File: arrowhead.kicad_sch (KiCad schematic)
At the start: 148 parts, among them J1 USB_C_Receptacle_USB2.0_14P, J2 USB_C_Receptacle_USB2.0_14P, J3 USB3_A, J4 USB3_A, U1 TUSB2046BVF, Y1 Crystal_GND23

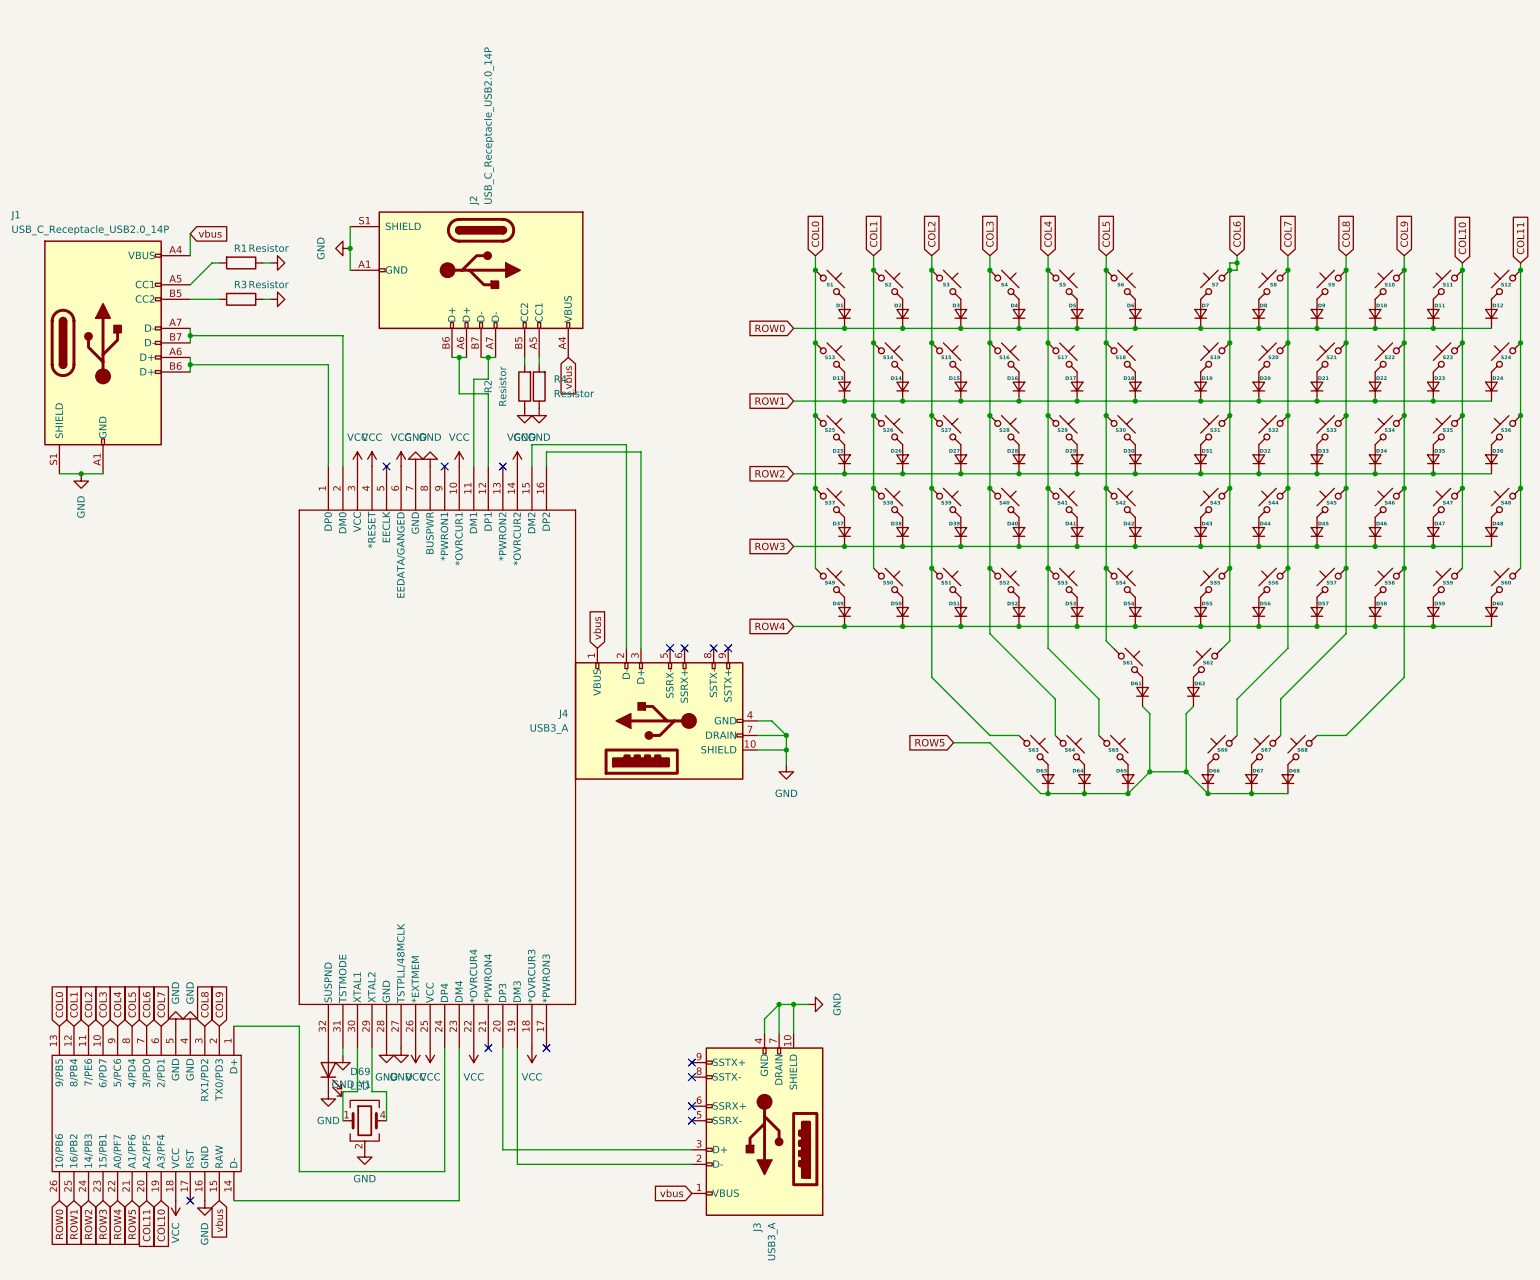
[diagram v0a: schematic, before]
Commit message: production run 1
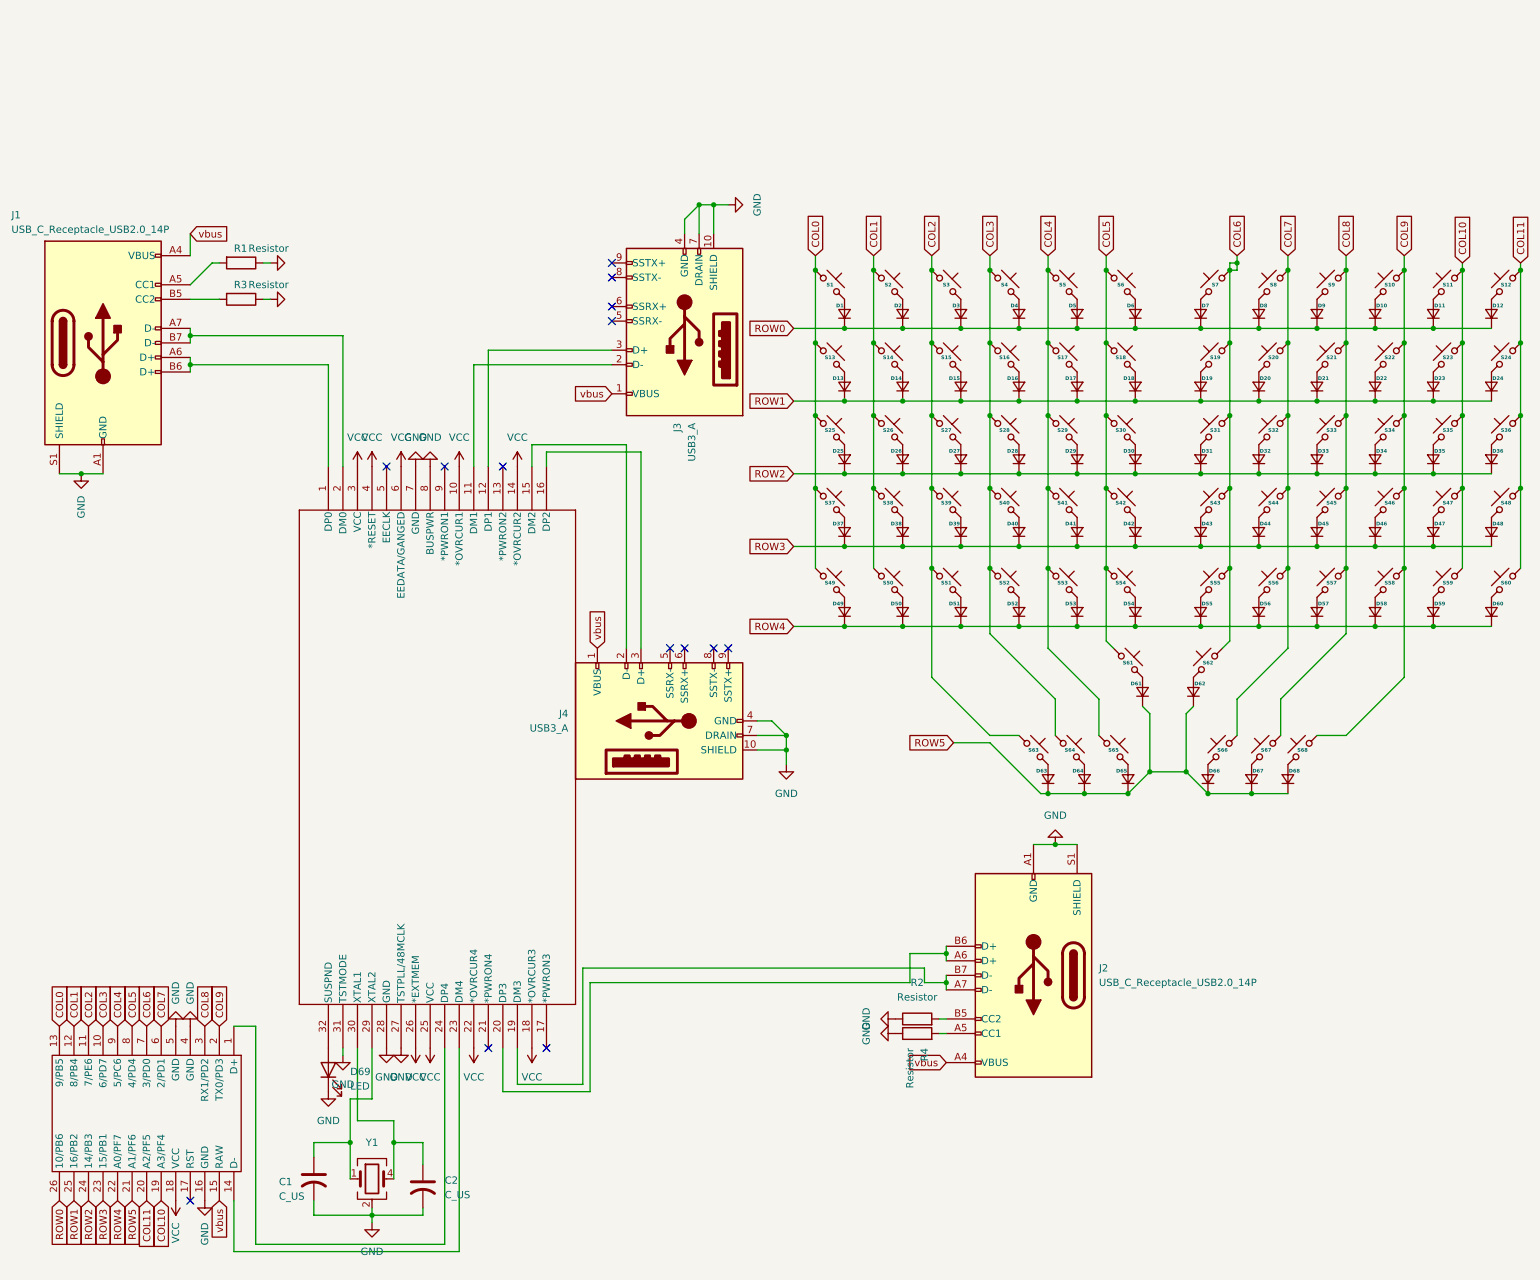
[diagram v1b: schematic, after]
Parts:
- added C1, C2: C_US, Capacitor_SMD:C_0603_1608Metric_Pad1.08x0.95mm_HandSolder, symbol Device:C_US
- D1, D10, D11, D12, D13, D14, D15, D16, D17, D18, D19, D2, D20, D21, D22, D23, D24, D25, D26, D27, D28, D29, D3, D30, D31, D32, D33, D34, D35, D36, D37, D38, D39, D4, D40, D41, D42, D43, D44, D45, D46, D47, D48, D49, D5, D50, D51, D52, D53, D54, D55, D56, D57, D58, D59, D6, D60, D61, D62, D63, D64, D65, D66, D67, D68, D7, D8, D9, S1, S10, S11, S12, S13, S14, S15, S16, S17, S18, S19, S2, S20, S21, S22, S23, S24, S25, S26, S27, S28, S29, S3, S30, S31, S32, S33, S34, S35, S36, S37, S38, S39, S4, S40, S41, S42, S43, S44, S45, S46, S47, S48, S49, S5, S50, S51, S52, S53, S54, S55, S56, S57, S58, S59, S6, S60, S61, S62, S63, S64, S65, S66, S67, S68, S7, S8, S9, U2: value ~ -> (none)
- D69: footprint LED_SMD:LED_0201_0603Metric -> LED_SMD:LED_0603_1608Metric_Pad1.05x0.95mm_HandSolder
- Y1: footprint Crystal:Crystal_SMD_7050-2Pin_7.0x5.0mm -> Crystal:Crystal_SMD_7050-4Pin_7.0x5.0mm
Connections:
- net GND: now also C1.2, C2.2
- net at Y1.1: now also U1.29 (XTAL2), C1.1; no longer U1.30 (XTAL1)
- net at Y1.4: now also U1.30 (XTAL1), C2.1; no longer U1.29 (XTAL2)
- net at J2.A7 (D-), J2.B7 (D-): now also U1.19 (DM3); no longer U1.11 (DM1)
- net at J2.A6 (D+), J2.B6 (D+): now also U1.20 (DP3); no longer U1.12 (DP1)
- net at J3.2 (D-): now also U1.11 (DM1); no longer U1.19 (DM3)
- net at J3.3 (D+): now also U1.12 (DP1); no longer U1.20 (DP3)
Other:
- moved on the sheet: J2, J3, R2, R4, Y1
